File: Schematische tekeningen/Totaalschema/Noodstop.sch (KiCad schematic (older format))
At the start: 19 parts, among them J8 Noodstop, Q4 BS170, Q5 BS170, U11 PC817, U12 PC817, U13 74AHC1G32

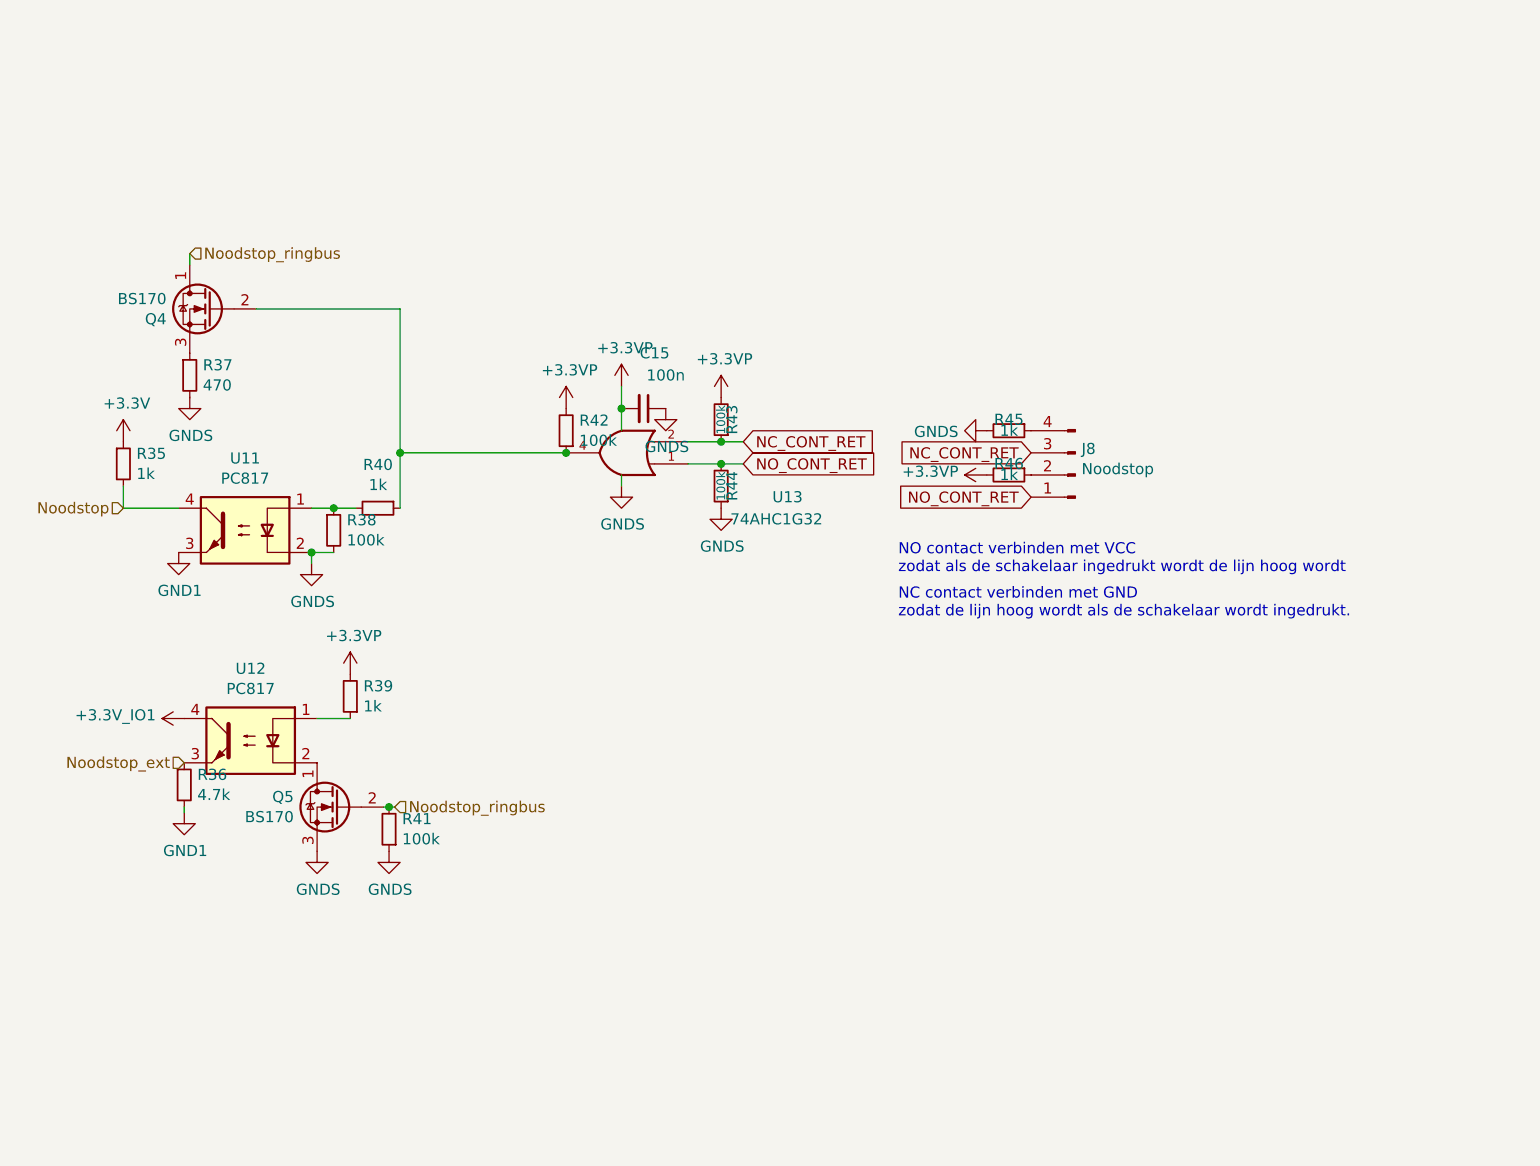
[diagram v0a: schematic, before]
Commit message: Totaalschema in orde maken
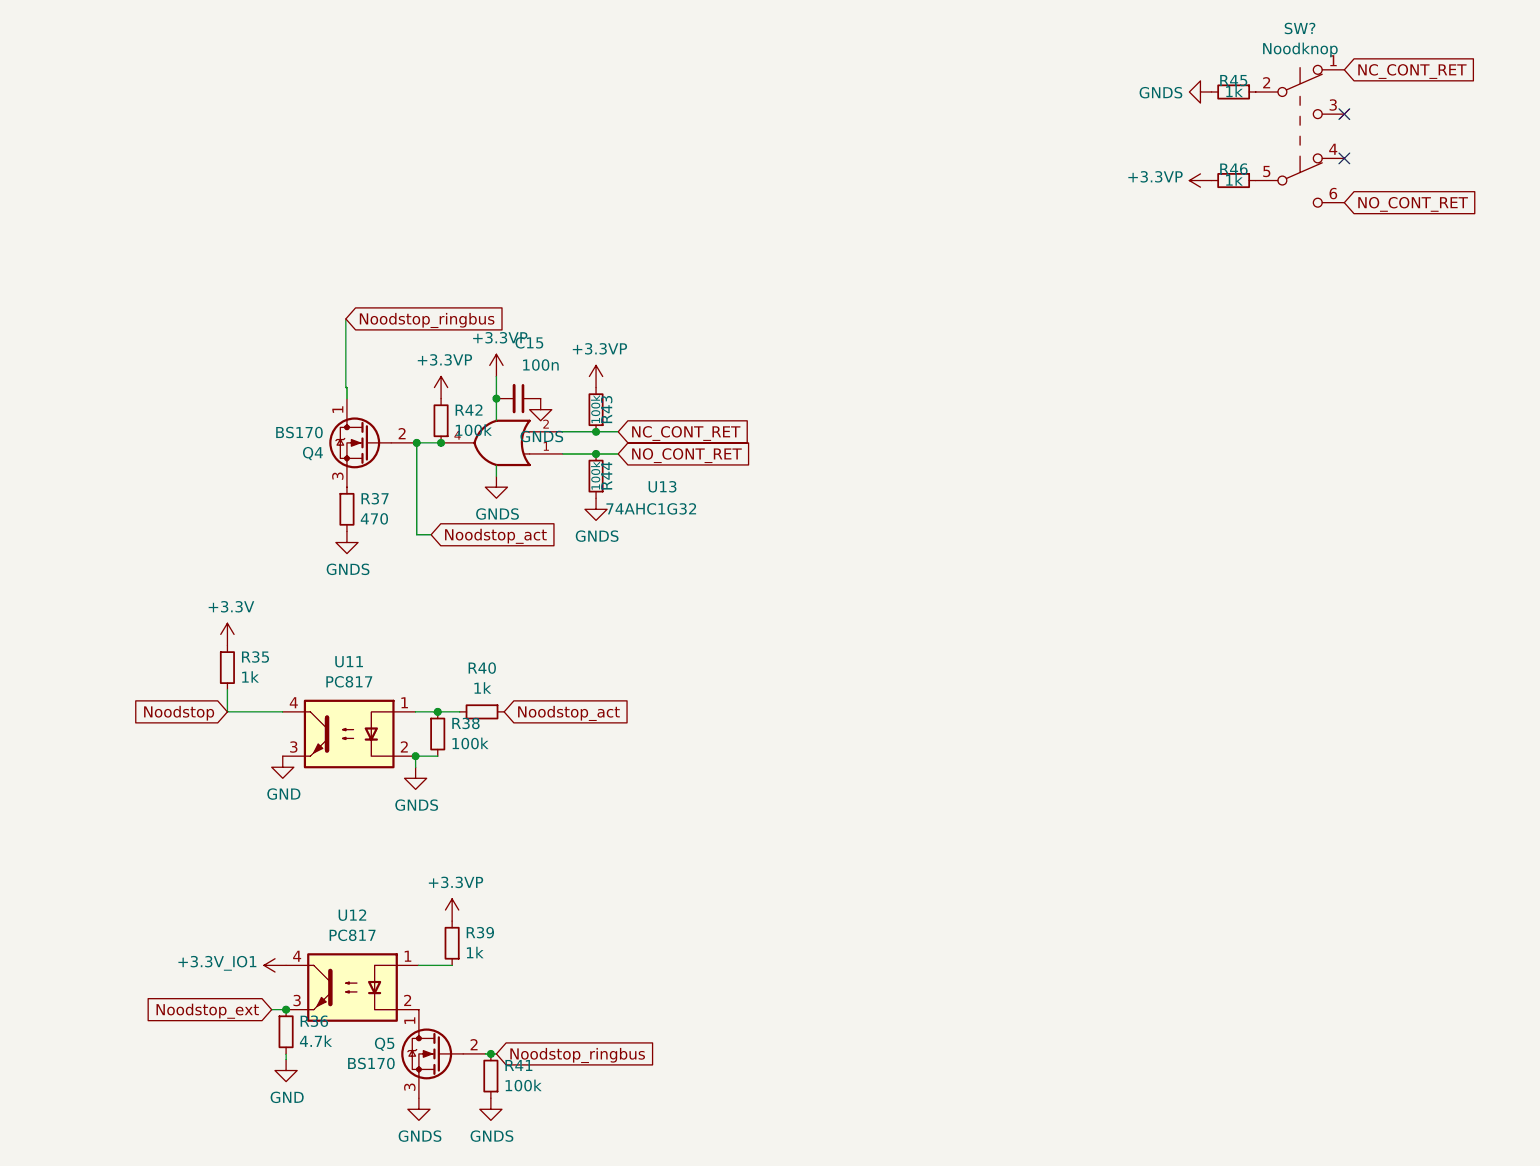
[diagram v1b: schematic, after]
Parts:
- removed J8: Noodstop, Connector_PinHeader_2.54mm:PinHeader_1x04_P2.54mm_Vertical, symbol Connector:Conn_01x04_Male
- added SW?: Noodknop, symbol Switch:SW_Push_DPDT
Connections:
- net GND1 is gone; now on net +3.3VP: R36.2, U11.3
- net NC_CONT_RET: now also SW?.1 (A)
- net NO_CONT_RET: now also SW?.6 (C)
- net Noodstop_act: now reaches Q4.2 (G), R40.1, R42.1, U13.4
- net at R46.1: now also SW?.5 (B)
- net at R45.1: now also SW?.2 (B)
- no-connect marks 0 -> 2
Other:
- note removed: "NC contact verbinden met GND \nzodat de lijn hoog wordt als de schakelaar wordt ingedrukt."
- note removed: "NO contact verbinden met VCC\nzodat als de schakelaar ingedrukt wordt de lijn hoog wordt"
- moved on the sheet: C15, Q4, Q5, R35, R36, R37, R38, R39, R40, R41, R42, R43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
